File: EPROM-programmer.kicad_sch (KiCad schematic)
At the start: 2 parts, among them U1 ATmega1284-P, U2 MCP2221AxP

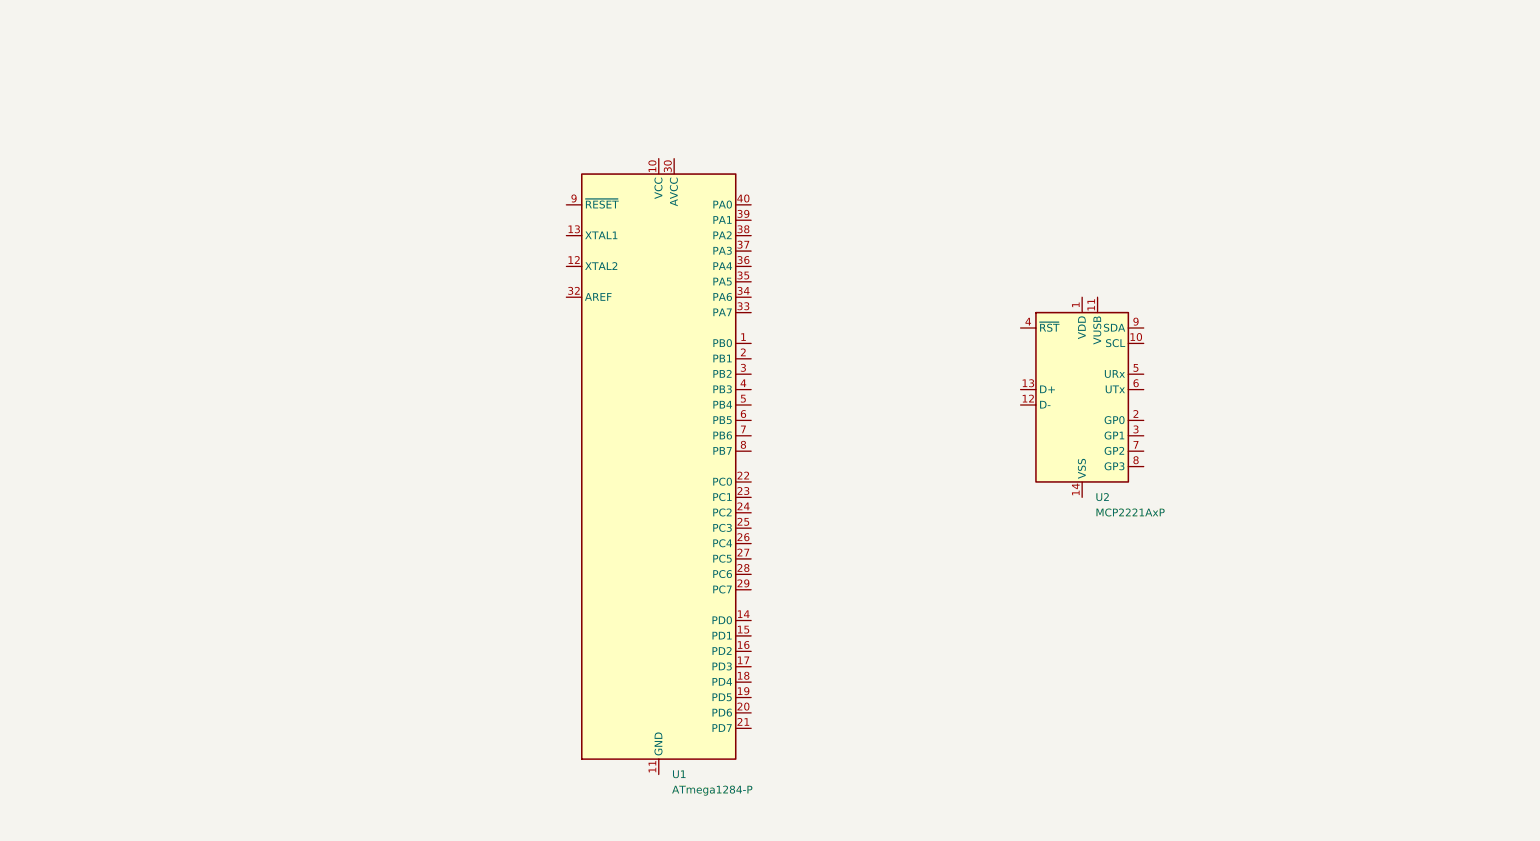
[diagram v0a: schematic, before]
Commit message: Some initial stuff
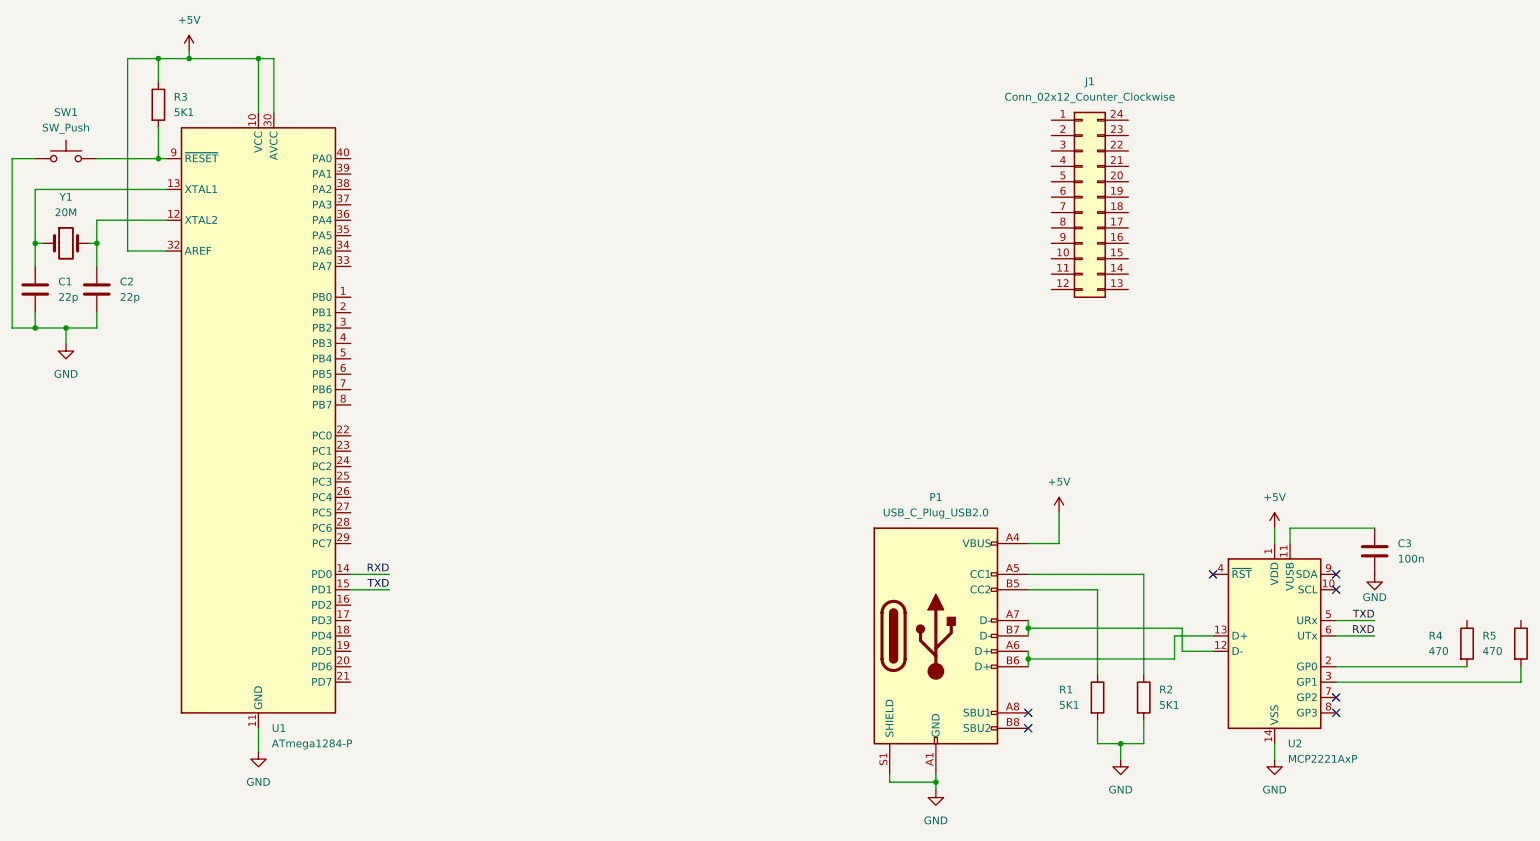
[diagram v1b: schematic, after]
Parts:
- added C1, C2: 22p, Capacitor_THT:C_Rect_L4.6mm_W3.0mm_P2.50mm_MKS02_FKP02, symbol Device:C
- added C3: 100n, Capacitor_THT:C_Rect_L4.6mm_W3.0mm_P2.50mm_MKS02_FKP02, symbol Device:C
- added J1: Conn_02x12_Counter_Clockwise, Local:DIP_Socket-24_W11.9_W12.7_W15.24_W17.78_W18.5_3M_224-1275-00-0602J, symbol Connector_Generic:Conn_02x12_Counter_Clockwise
- added P1: USB_C_Plug_USB2.0, Connector_USB:USB_C_Receptacle_GCT_USB4085, symbol Connector:USB_C_Receptacle_USB2.0
- added R1, R2, R3: 5K1, Resistor_THT:R_Axial_DIN0207_L6.3mm_D2.5mm_P10.16mm_Horizontal, symbol Device:R
- added R4, R5: 470, Resistor_THT:R_Axial_DIN0207_L6.3mm_D2.5mm_P10.16mm_Horizontal, symbol Device:R
- added SW1: SW_Push, symbol Switch:SW_Push
- added Y1: 20M, Crystal:Crystal_HC49-U_Vertical, symbol Device:Crystal
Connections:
- net +5V: now reaches U2.1 (VDD)
- net +5V: now also U1.10 (VCC), U1.30 (AVCC), U1.32 (AREF), P1.A4 (VBUS), P1.A9 (VBUS), P1.B4 (VBUS), P1.B9 (VBUS), R3.1
- net at U2.11 (VUSB): now also C3.1
- net at U2.12 (D-): now also P1.A7 (D-), P1.B7 (D-)
- net at U2.13 (D+): now also P1.A6 (D+), P1.B6 (D+)
- net GND: now reaches U2.14 (VSS)
- net GND: now also U1.11 (GND), U1.31 (GND), C1.2, C2.2, C3.2, P1.A1 (GND), P1.A12 (GND), P1.B1 (GND), P1.B12 (GND), P1.S1 (SHIELD), R1.2, R2.2, SW1.1
- net at U2.2 (GP0): now also R4.2
- net at U2.3 (GP1): now also R5.2
- net TXD: now reaches U2.5 (URx)
- net TXD: now also U1.15 (PD1)
- net RXD: now reaches U2.6 (UTx)
- net RXD: now also U1.14 (PD0)
- net at U1.12 (XTAL2): now also C2.1, Y1.2
- net at U1.13 (XTAL1): now also C1.1, Y1.1
- net at U1.9 (~{RESET}): now also R3.2, SW1.2
- new net: P1.A5 (CC1), R2.1
- new net: P1.B5 (CC2), R1.1
- no-connect marks 0 -> 7
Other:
- moved on the sheet: U1, U2
